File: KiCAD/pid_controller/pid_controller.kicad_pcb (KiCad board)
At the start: 2 copper layers, 121.6 x 61.3 mm, 37 parts, among them J1 12VDC Power In, J2 Heater, J4 Rotary Encoder, Q1 irf3205/2SK3570/IPB11N03LA, Q2 N.A, U1 L7805, U2 LM35-LP, U3 MT3608, U4 CAT24C128, U5 PS2561/PC817

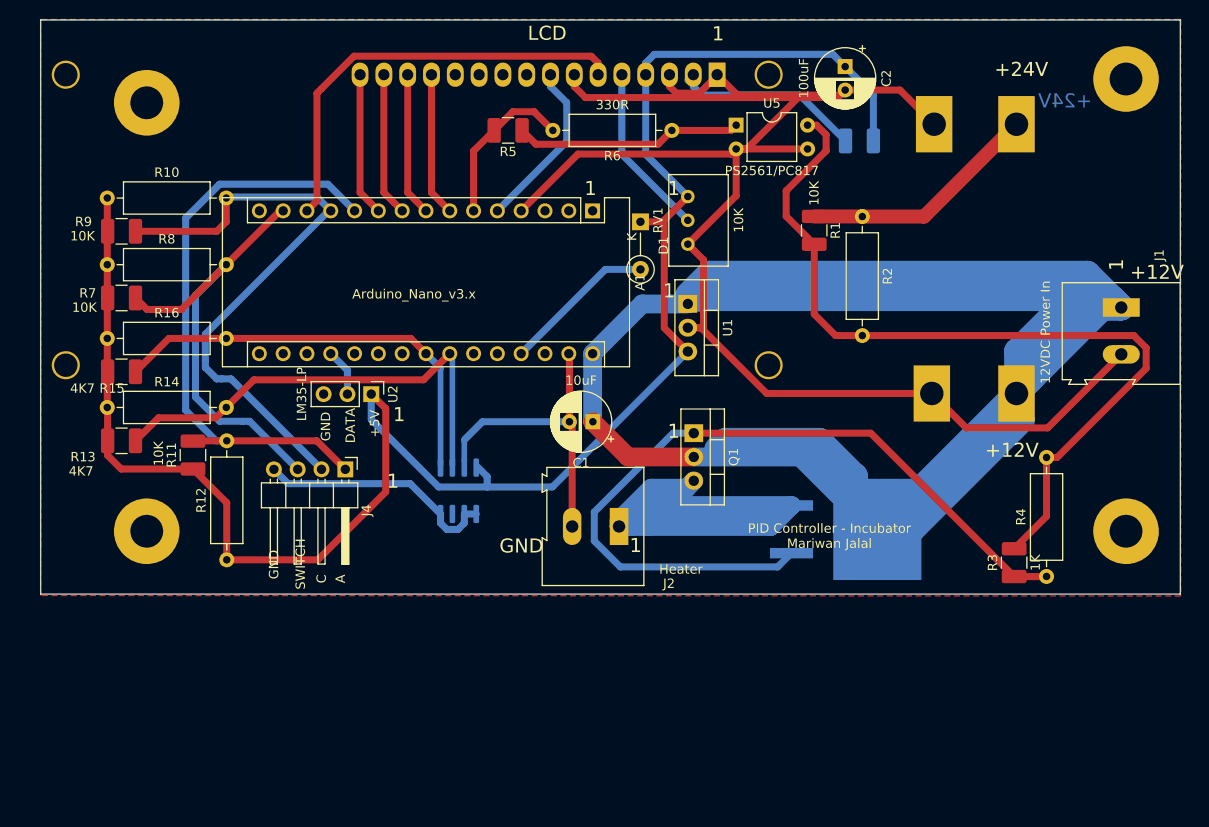
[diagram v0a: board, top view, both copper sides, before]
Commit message: Redesign the PCB and add some other footprints
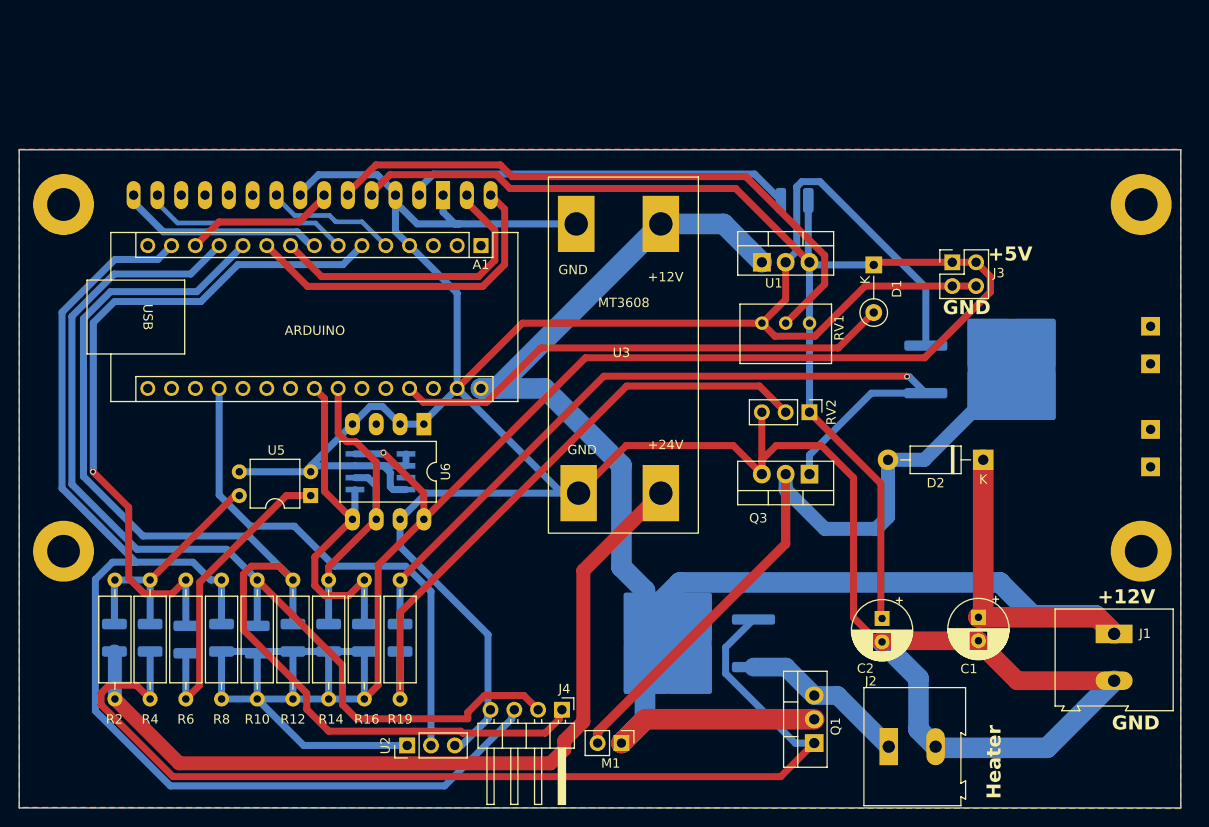
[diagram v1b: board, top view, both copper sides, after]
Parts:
- removed Hole1, Hole2, Hole3, Hole4: MountingHole_3.5mm_Pad, MountingHole:MountingHole_3.5mm_Pad
- added D2: 1N4001, Diode_THT:D_DO-41_SOD81_P10.16mm_Horizontal, F.Cu at (177.8, 101.6)
- added J3: +5V, Connector_PinHeader_2.54mm:PinHeader_2x02_P2.54mm_Vertical, F.Cu at (174.5, 80.5)
- added M1: Fan, Connector_PinHeader_2.54mm:PinHeader_1x02_P2.54mm_Vertical, F.Cu at (139.2, 131.8)
- added Q3: irf3205/2SK3570/IPB11N03LA, Package_TO_SOT_THT:TO-220-3_Vertical, F.Cu at (159.3, 103.1)
- added Q4: N.A, Package_TO_SOT_SMD:TO-263-2, B.Cu at (179.3, 91.9)
- added R18: N.A, Resistor_SMD:R_1210_3225Metric, B.Cu at (115.6, 120.6)
- added R19: 1K, Resistor_THT:R_Axial_DIN0309_L9.0mm_D3.2mm_P12.70mm_Horizontal, F.Cu at (115.6, 127.1)
- added RV2: 5K, Connector_PinHeader_2.54mm:PinHeader_1x03_P2.54mm_Vertical, F.Cu at (159.3, 96.5)
- added U6: 24LC64, Package_DIP:DIP-8_W10.16mm_LongPads, F.Cu at (118.1, 97.8)
- DS1: footprint Display:WC1602A -> Display:LCD-016N002L
- R1, R11, R13, R15, R3, R5, R7, R9: footprint Resistor_SMD:R_1210_3225Metric_Pad1.42x2.65mm_HandSolder -> Resistor_SMD:R_1210_3225Metric; moved to B.Cu
- R17: footprint Resistor_SMD:R_1210_3225Metric_Pad1.42x2.65mm_HandSolder -> Resistor_SMD:R_1210_3225Metric
- R6: value 330R -> 1K
- U3: moved to F.Cu
- U4: footprint Package_SO:SOIC-8_3.9x4.9mm_P1.27mm -> Package_SO:PowerIntegrations_SO-8
- U5: value PS2561/PC817 -> PS2561
- moved R4 96.5 mm to (88.9, 127.1)
- moved R2 94.9 mm to (85.1, 127.1), turned to 90 degrees
- moved R3 92.5 mm to (88.9, 120.6)
- moved R1 86.4 mm to (85.1, 120.6), turned to 90 degrees
- moved R6 79.8 mm to (92.7, 127.1), turned to 90 degrees
- moved R5 64.3 mm to (92.7, 120.8), turned to 90 degrees
- moved U5 60.2 mm to (106.0, 105.4), turned to 180 degrees
- moved C2 59.0 mm to (167.0, 118.5)
- moved R10 55.8 mm to (100.3, 127.1), turned to 90 degrees
- moved R8 47.9 mm to (96.5, 127.1), turned to 90 degrees
- moved R16 47.3 mm to (111.8, 127.1), turned to 90 degrees
- moved C1 46.1 mm to (177.3, 118.4), turned to -90 degrees
- moved R9 45.9 mm to (100.3, 120.8), turned to 90 degrees
- moved U3 39.2 mm to (152.4, 90.4), turned to -90 degrees
- moved R14 39.1 mm to (108.0, 127.1), turned to 90 degrees
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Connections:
- A1 pad 1: Net-(A1-Pad1) -> unconnected-(A1-D1/TX-Pad1)
- A1 pad 15: Net-(A1-Pad15) -> unconnected-(A1-D12-Pad15)
- A1 pad 16: Net-(A1-Pad16) -> unconnected-(A1-D13-Pad16)
- A1 pad 17: Net-(A1-Pad17) -> unconnected-(A1-3V3-Pad17)
- A1 pad 18: Net-(A1-Pad18) -> unconnected-(A1-AREF-Pad18)
- A1 pad 2: Net-(A1-Pad2) -> unconnected-(A1-D0/RX-Pad2)
- A1 pad 20: Net-(A1-Pad20) -> unconnected-(A1-A1-Pad20)
- A1 pad 21: Net-(A1-Pad21) -> unconnected-(A1-A2-Pad21)
- A1 pad 22: Net-(A1-Pad22) -> unconnected-(A1-A3-Pad22)
- A1 pad 25: Net-(A1-Pad25) -> unconnected-(A1-A6-Pad25)
- A1 pad 26: Net-(A1-Pad26) -> unconnected-(A1-A7-Pad26)
- A1 pad 28: Net-(A1-Pad28) -> unconnected-(A1-~{RESET}-Pad28)
- A1 pad 3: Net-(A1-Pad3) -> unconnected-(A1-~{RESET}-Pad3)
- DS1 pad 10: Net-(DS1-Pad10) -> unconnected-(DS1-DB1-Pad10)
- DS1 pad 11: Net-(DS1-Pad11) -> unconnected-(DS1-DB2-Pad11)
- DS1 pad 12: Net-(DS1-Pad12) -> unconnected-(DS1-DB3-Pad12)
- DS1 pad 9: Net-(DS1-Pad9) -> unconnected-(DS1-DB0-Pad9)
- U4 pad 3: Net-(U4-Pad3) -> unconnected-(U4-A2-Pad3)
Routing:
- net GND: track 242.8 -> 401.7 mm
- net +5V: track 196.2 -> 299.3 mm, vias 0 -> 1
- net Net-(Q3-G): track 0.00 -> 87.7 mm, vias 0 -> 1
- net /ROTARY_SWITCH: track 50.2 -> 130.4 mm
- net Net-(D2-A): track 0.00 -> 71.6 mm
- net +12V: track 263.0 -> 193.2 mm
- net /PWM: track 0.00 -> 66.6 mm
- net Net-(R1-Pad2): track 89.4 -> 26.4 mm
- net +24V: track 25.7 -> 88.1 mm
- net /A: track 64.5 -> 121.9 mm
- net PWM_Signal: track 17.4 -> 73.2 mm, vias 0 -> 1
- net Net-(A1-A0): track 5.05 -> 54.7 mm
- net /HeaterPowerOut: track 65.9 -> 18.0 mm
- net Net-(DS1-Vo): track 18.5 -> 65.3 mm
- net /ROTARY_DATA: track 63.7 -> 106.3 mm
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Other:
- board size 121.6 x 61.3 mm -> 124 x 70.2 mm
- board text added: "ARDUINO"
- board text added: "Heater"
- board text removed: "1"
- board text removed: "A"
- board text removed: "C"
- board text removed: "DATA"
- board text removed: "LCD"
- board text removed: "PID Controller - Incubator Mariwan Jalal"
- board text removed: "SWITCH"
